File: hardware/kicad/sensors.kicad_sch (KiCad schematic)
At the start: 9 parts, among them J6 Qwiic, U4 LSM6DSOTR, U5 MAX17048G+

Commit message: move components to use bwlc1a library
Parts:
- J6: footprint Connector_JST:JST_SH_SM04B-SRSS-TB_1x04-1MP_P1.00mm_Horizontal -> bwlc1a:JST_SH_SM04B-SRSS-TB_1x04-1MP_P1.00mm_Horizontal
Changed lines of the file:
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@@
 			)
 		)
-		(property "Footprint" "Connector_JST:JST_SH_SM04B-SRSS-TB_1x04-1MP_P1.00mm_Horizontal"
+		(property "Footprint" "bwlc1a:JST_SH_SM04B-SRSS-TB_1x04-1MP_P1.00mm_Horizontal"
 			(at 179.07 122.555 0)
 			(effects

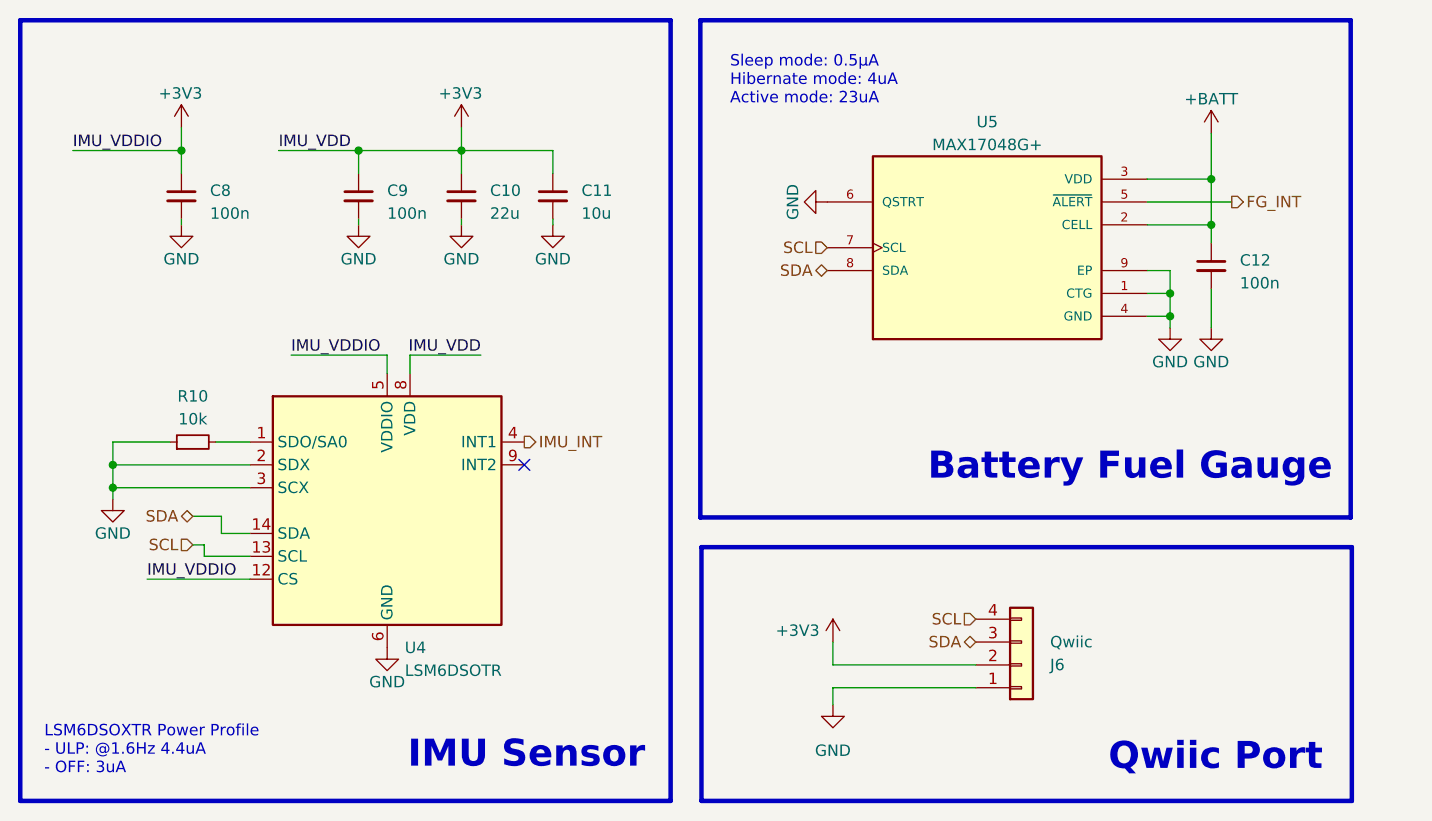
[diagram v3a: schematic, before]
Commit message: update bill of materials
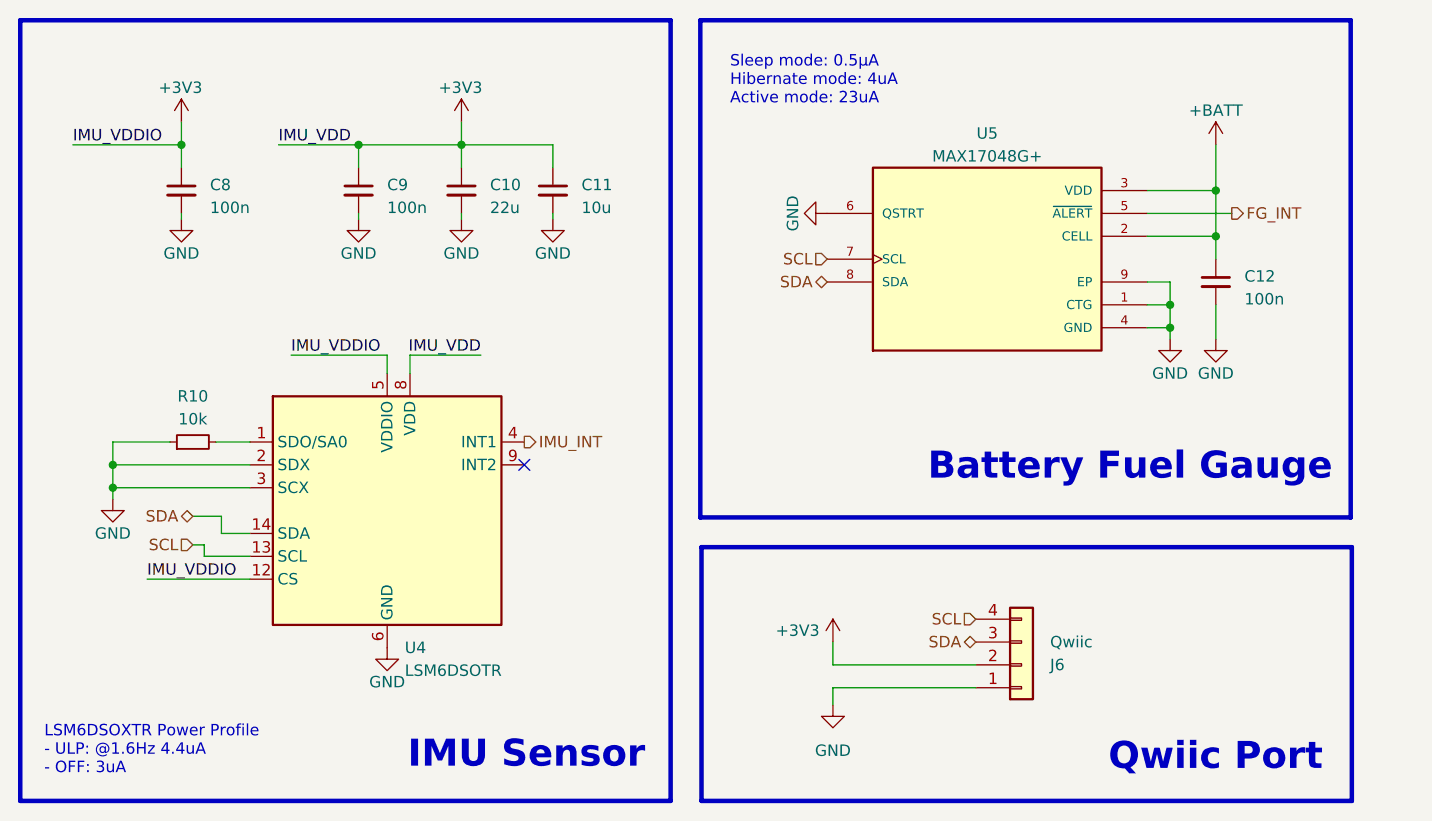
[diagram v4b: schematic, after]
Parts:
- C10: Id 4 -> (none); Manufacture Samsung Electro-Mechanics -> (none); Manufacture Part Number CL10A226MP8NUNE -> (none); Manufacturer (none) -> Samsung Electro-Mechanics; Manufacturer Part Number (none) -> CL10A226MP8NUNE; Type SMD -> (none)
- C11: Id 1 -> (none); Manufacture Samsung Electro-Mechanics -> (none); Manufacture Part Number CL10A106KP8NNNC -> (none); Manufacturer (none) -> Samsung Electro-Mechanics; Manufacturer Part Number (none) -> CL10A106KP8NNNC; Type SMD -> (none)
- C12, C8, C9: Id 3 -> (none); Manufacture Samsung Electro-Mechanics -> (none); Manufacture Part Number CL05B104KO5NNNC -> (none); Manufacturer (none) -> Samsung Electro-Mechanics; Manufacturer Part Number (none) -> CL05B104KO5NNNC; Type SMD -> (none)
- J6: Distributor (none) -> LCSC; Distributor Link (none) -> https://www.lcsc.com/product-detail/Wire-To-Board-Wire-To-W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; Distributor Part Number (none) -> C160404; Manufacturer JST Sales America -> JST; Manufacturer Part Number (none) -> SM04B-SRSS-TB(LF)(SN); Part Number SM04B-SRSS-TB -> (none)
- R10: Id 40 -> (none); Manufacture UNI-ROYAL(Uniroyal Elec) -> (none); Manufacture Part Number 0402WGF1002TCE -> (none); Manufacturer (none) -> UNI-ROYAL(Uniroyal Elec); Manufacturer Part Number (none) -> 0402WGF1002TCE; Type SMD -> (none)
- U4: Distributor Link https://datasheet.lcsc.com/lcsc/2108070730_STMicroelectroni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 -> https://www.lcsc.com/product-detail/Attitude-Sensor-Gyrosco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; Part Description LGA-14 Attitude Sensor/Gyroscope ROHS -> (none)
- U5: Id 54 -> (none); Manufacture Analog Devices Inc./Maxim Integrated -> (none); Manufacture Part Number MAX17048G+T10 -> (none); Manufacturer (none) -> Analog Devices Inc./Maxim Integrated; Manufacturer Part Number (none) -> MAX17048G+T10; Type SMD -> (none)
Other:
- moved on the sheet: C10, C11, C8, U5
